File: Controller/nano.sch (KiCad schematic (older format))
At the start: 24 parts, among them J10 ICSP, J15 UJ2-BH-1-TH, K1 SW_RESET, U2 INTERFACE-CH340T_SSOP20_, U3 MCU-ATMEGA328P-AU_TQFP32_, Y1 12MHz, Y2 16MHZ

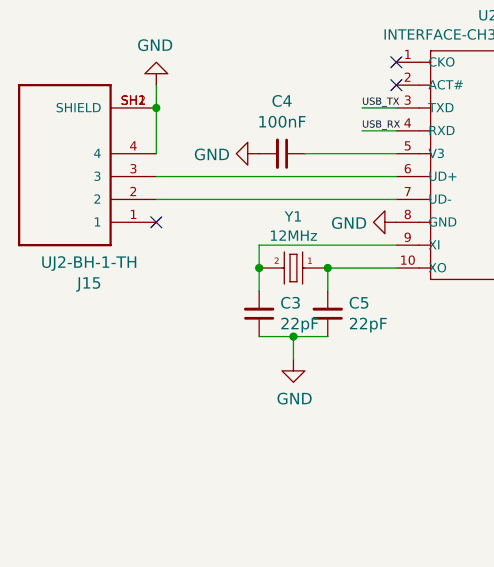
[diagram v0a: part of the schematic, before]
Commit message: Mostly final layout
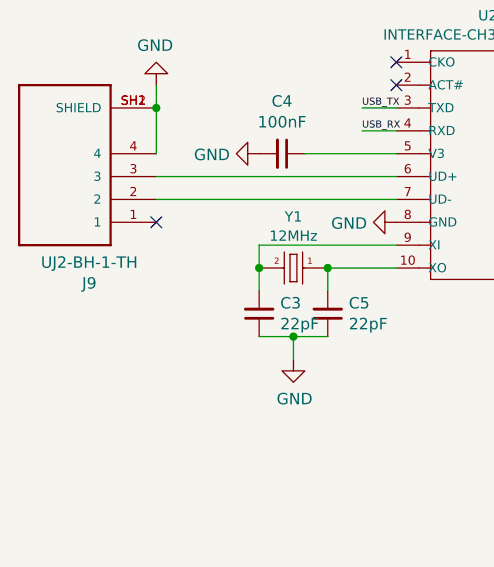
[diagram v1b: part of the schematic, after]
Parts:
- renumbered J15 to J9
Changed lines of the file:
@@
 RST
 $Comp
-L UJ2-BH-1-TH:UJ2-BH-1-TH J15
+L UJ2-BH-1-TH:UJ2-BH-1-TH J9
 U 1 1 5D55598E
 P 3300 2150
-F 0 "J15" H 3407 2617 50  0000 C CNN
+F 0 "J9" H 3407 2617 50  0000 C CNN
 F 1 "UJ2-BH-1-TH" H 3407 2526 50  0000 C CNN
 F 2 "CUI:CUI_UJ2-BH-1-TH" H 3300 2150 50  0001 L BNN
